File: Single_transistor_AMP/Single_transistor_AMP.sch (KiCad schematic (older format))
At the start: 10 parts, among them J1 ieeja, J2 Izeja, J3 Barosana, Q1 BC547

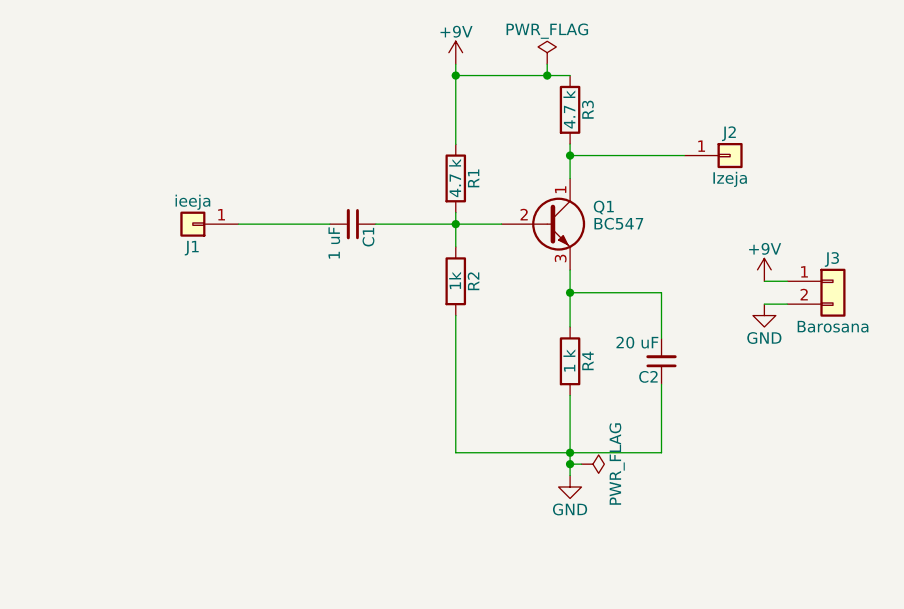
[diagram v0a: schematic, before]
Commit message: Majasdarbs peec 8. lekcijas, kur jauzzimee plate
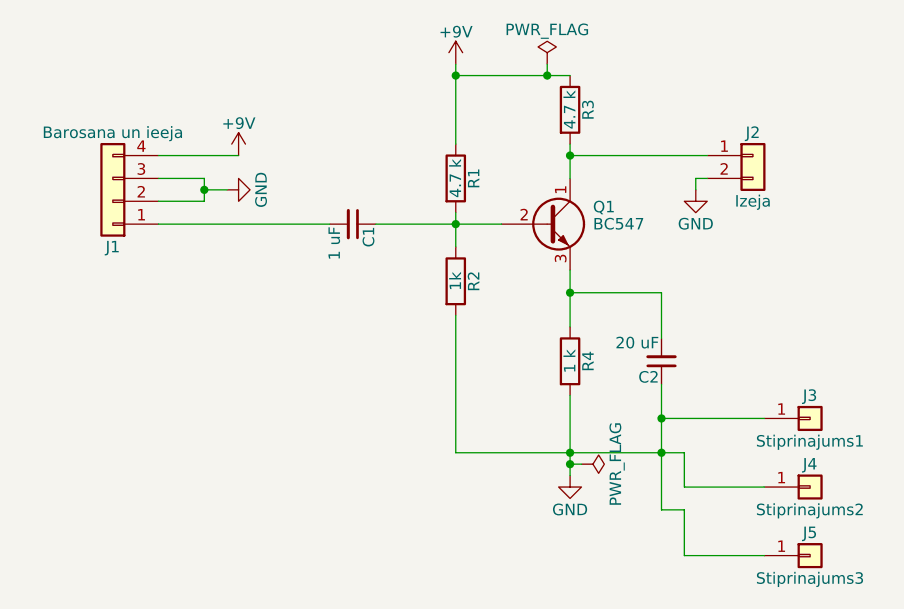
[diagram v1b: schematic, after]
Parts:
- removed J1: ieeja, Connectors:1pin, symbol Conn_01x01
- removed J2: Izeja, Connectors:1pin, symbol Conn_01x01
- removed J3: Barosana, Connectors:AK300-2, symbol Conn_01x02
- added J1: Barosana un ieeja, Connectors:AK300-4, symbol Conn_01x04
- added J2: Izeja, Connectors:AK300-2, symbol Conn_01x02
- added J3: Stiprinajums1, Mounting_Holes:MountingHole_2.2mm_M2_Pad, symbol Conn_01x01
- added J4: Stiprinajums2, Mounting_Holes:MountingHole_2.2mm_M2_Pad, symbol Conn_01x01
- added J5: Stiprinajums3, Mounting_Holes:MountingHole_2.2mm_M2_Pad, symbol Conn_01x01
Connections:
- net +9V: now also J1.4 (Pin_4)
- net GND: now also J1.2 (Pin_2), J1.3 (Pin_3), J2.2 (Pin_2), J3.1 (Pin_1), J4.1 (Pin_1), J5.1 (Pin_1)
- net at Q1.1 (C), R3.2: now also J2.1 (Pin_1)
- net at C1.2: now also J1.1 (Pin_1)
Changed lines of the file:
@@
 LIBS:contrib
 LIBS:valves
+LIBS:Single_transistor_AMP-cache
 EELAYER 25 0
 EELAYER END
@@
 Connection ~ 5600 3200
 Wire Wire Line
-	6000 3900 6000 3600
+	6000 3600 6000 4150
 Wire Wire Line
 	5600 3650 5600 4000
@@
 $EndComp
 Wire Wire Line
-	5100 3900 6000 3900
+	5100 3900 6100 3900
 Wire Wire Line
 	5100 3900 5100 3300
@@
 	5100 2250 5600 2250
 Wire Wire Line
-	5600 2600 6100 2600
+	5600 2600 6200 2600
 Connection ~ 5600 2600
 $Comp
@@
 Connection ~ 5100 2250
 Wire Wire Line
-	4150 2900 4550 2900
+	3800 2900 4550 2900
 $Comp
 L PWR_FLAG #FLG03
@@
 	5500 2250 5500 2200
 Connection ~ 5500 2250
-$Comp
-L Conn_01x01 J2
-U 1 1 5AAA46B5
-P 6300 2600
-F 0 "J2" H 6300 2700 50  0000 C CNN
-F 1 "Izeja" H 6300 2500 50  0000 C CNN
-F 2 "Connectors:1pin" H 6300 2600 50  0001 C CNN
-F 3 "https://eu.mouser.com/ds/2/181/M22-251-1134335.pdf" H 6300 2600 50  0001 C CNN
-	1    6300 2600
-	1    0    0    -1
-$EndComp
-$Comp
-L Conn_01x01 J1
-U 1 1 5AAA4731
-P 3950 2900
-F 0 "J1" H 3950 3000 50  0000 C CNN
-F 1 "ieeja" H 3950 2800 50  0000 C CNN
-F 2 "Connectors:1pin" H 3950 2900 50  0001 C CNN
-F 3 "https://eu.mouser.com/ds/2/181/M22-251-1134335.pdf" H 3950 2900 50  0001 C CNN
-	1    3950 2900
-	-1   0    0    1
-$EndComp
 $Comp
 L PWR_FLAG #FLG04
@@
 Connection ~ 5600 3950
 $Comp
-L Conn_01x02 J3
-U 1 1 5AAA4A96
-P 6750 3150
-F 0 "J3" H 6750 3250 50  0000 C CNN
-F 1 "Barosana" H 6750 2950 50  0000 C CNN
-F 2 "Connectors:AK300-2" H 6750 3150 50  0001 C CNN
-F 3 "http://www.fastelettronica.com/PTR_morsetti.pdf" H 6750 3150 50  0001 C CNN
-	1    6750 3150
-	1    0    0    -1
-$EndComp
-$Comp
-L +9V #PWR05
-U 1 1 5AAA4AF5
-P 6450 3150
-F 0 "#PWR05" H 6450 3000 50  0001 C CNN
-F 1 "+9V" H 6450 3290 50  0000 C CNN
-F 2 "" H 6450 3150 50  0001 C CNN
-F 3 "" H 6450 3150 50  0001 C CNN
-	1    6450 3150
-	1    0    0    -1
-$EndComp
+L Conn_01x02 J2
+U 1 1 5ADF7E08
+P 6400 2600
+F 0 "J2" H 6400 2700 50  0000 C CNN
+F 1 "Izeja" H 6400 2400 50  0000 C CNN
+F 2 "Connectors:AK300-2" H 6400 2600 50  0001 C CNN
+F 3 "https://eu.mouser.com/datasheet/2/16/PCBMETRC-24178.pdf" H 6400 2600 50  0001 C CNN
+	1    6400 2600
+	1    0    0    -1
+$EndComp
+$Comp
+L GND #PWR05
+U 1 1 5ADF7EF4
+P 6150 2750
+F 0 "#PWR05" H 6150 2500 50  0001 C CNN
+F 1 "GND" H 6150 2600 50  0000 C CNN
+F 2 "" H 6150 2750 50  0001 C CNN
+F 3 "" H 6150 2750 50  0001 C CNN
+	1    6150 2750
+	1    0    0    -1
+$EndComp
+Wire Wire Line
+	6200 2700 6150 2700
+Wire Wire Line
+	6150 2700 6150 2750
+$Comp
+L Conn_01x04 J1
+U 1 1 5ADF7F72
+P 3600 2800
+F 0 "J1" H 3600 3000 50  0000 C CNN
+F 1 "Barosana un ieeja" H 3600 2500 50  0000 C CNN
+F 2 "Connectors:AK300-4" H 3600 2800 50  0001 C CNN
+F 3 "https://www.alliedelec.com/m/d/5562820d7d96e18ed6aa6b65b62d0d03.pdf" H 3600 2800 50  0001 C CNN
+	1    3600 2800
+	-1   0    0    1
+$EndComp
+Wire Wire Line
+	3800 2800 4000 2800
+Wire Wire Line
+	4000 2800 4000 2700
+Wire Wire Line
+	4000 2700 3800 2700
 $Comp
 L GND #PWR06
-U 1 1 5AAA4B1D
-P 6450 3250
-F 0 "#PWR06" H 6450 3000 50  0001 C CNN
-F 1 "GND" H 6450 3100 50  0000 C CNN
-F 2 "" H 6450 3250 50  0001 C CNN
-F 3 "" H 6450 3250 50  0001 C CNN
-	1    6450 3250
-	1    0    0    -1
-$EndComp
-Wire Wire Line
-	6550 3150 6450 3150
-Wire Wire Line
-	6550 3250 6450 3250
+U 1 1 5ADF80F6
+P 4100 2750
+F 0 "#PWR06" H 4100 2500 50  0001 C CNN
+F 1 "GND" H 4100 2600 50  0000 C CNN
+F 2 "" H 4100 2750 50  0001 C CNN
+F 3 "" H 4100 2750 50  0001 C CNN
+	1    4100 2750
+	0    -1   -1   0
+$EndComp
+Wire Wire Line
+	4100 2750 4000 2750
+Connection ~ 4000 2750
+$Comp
+L +9V #PWR07
+U 1 1 5ADF8144
+P 4150 2600
+F 0 "#PWR07" H 4150 2450 50  0001 C CNN
+F 1 "+9V" H 4150 2740 50  0000 C CNN
+F 2 "" H 4150 2600 50  0001 C CNN
+F 3 "" H 4150 2600 50  0001 C CNN
+	1    4150 2600
+	1    0    0    -1
+$EndComp
+Wire Wire Line
+	3800 2600 4150 2600
+$Comp
+L Conn_01x01 J3
+U 1 1 5ADF8EFF
+P 6650 3750
+F 0 "J3" H 6650 3850 50  0000 C CNN
+F 1 "Stiprinajums1" H 6650 3650 50  0000 C CNN
+F 2 "Mounting_Holes:MountingHole_2.2mm_M2_Pad" H 6650 3750 50  0001 C CNN
+F 3 "" H 6650 3750 50  0001 C CNN
+	1    6650 3750
+	1    0    0    -1
+$EndComp
+$Comp
+L Conn_01x01 J4
+U 1 1 5ADF8F56
+P 6650 4050
+F 0 "J4" H 6650 4150 50  0000 C CNN
+F 1 "Stiprinajums2" H 6650 3950 50  0000 C CNN
+F 2 "Mounting_Holes:MountingHole_2.2mm_M2_Pad" H 6650 4050 50  0001 C CNN
+F 3 "" H 6650 4050 50  0001 C CNN
+	1    6650 4050
+	1    0    0    -1
+$EndComp
+$Comp
+L Conn_01x01 J5
+U 1 1 5ADF8F8B
+P 6650 4350
+F 0 "J5" H 6650 4450 50  0000 C CNN
+F 1 "Stiprinajums3" H 6650 4250 50  0000 C CNN
+F 2 "Mounting_Holes:MountingHole_2.2mm_M2_Pad" H 6650 4350 50  0001 C CNN
+F 3 "" H 6650 4350 50  0001 C CNN
+	1    6650 4350
+	1    0    0    -1
+$EndComp
+Wire Wire Line
+	6000 3750 6450 3750
+Connection ~ 6000 3750
+Wire Wire Line
+	6100 3900 6100 4050
+Connection ~ 6000 3900
+Wire Wire Line
+	6000 4150 6100 4150
+Wire Wire Line
+	6100 4050 6450 4050
+Wire Wire Line
+	6100 4150 6100 4350
+Wire Wire Line
+	6100 4350 6450 4350
 $EndSCHEMATC

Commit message: Single_transistor_AMP 2. iteraacija
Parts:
- C1: footprint Capacitors_THT:CP_Axial_L10.0mm_D4.5mm_P15.00mm_Horizontal -> Capacitors_THT:C_Rect_L10.0mm_W2.5mm_P7.50mm_MKS4
- C2: footprint Capacitors_THT:CP_Radial_D10.0mm_P2.50mm -> Capacitors_THT:C_Rect_L10.0mm_W2.5mm_P7.50mm_MKS4
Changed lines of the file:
@@
 F 0 "C1" H 4660 2970 50  0000 L CNN
 F 1 "1 uF" H 4660 2820 50  0000 L CNN
-F 2 "Capacitors_THT:CP_Axial_L10.0mm_D4.5mm_P15.00mm_Horizontal" H 4650 2900 50  0001 C CNN
+F 2 "Capacitors_THT:C_Rect_L10.0mm_W2.5mm_P7.50mm_MKS4" H 4650 2900 50  0001 C CNN
 F 3 "https://eu.mouser.com/ds/2/40/spingrd-776981.pdf" H 4650 2900 50  0001 C CNN
 	1    4650 2900
@@
 F 0 "C2" H 6010 3570 50  0000 L CNN
 F 1 "20 uF" H 6010 3420 50  0000 L CNN
-F 2 "Capacitors_THT:CP_Radial_D10.0mm_P2.50mm" H 6000 3500 50  0001 C CNN
+F 2 "Capacitors_THT:C_Rect_L10.0mm_W2.5mm_P7.50mm_MKS4" H 6000 3500 50  0001 C CNN
 F 3 "https://eu.mouser.com/ds/2/281/c49e-506.pdf" H 6000 3500 50  0001 C CNN
 	1    6000 3500
